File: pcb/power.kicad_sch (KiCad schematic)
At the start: 12 parts, among them P1 USB_C_Plug_USB2.0, U4 AZ1117IH-3.3TRG1

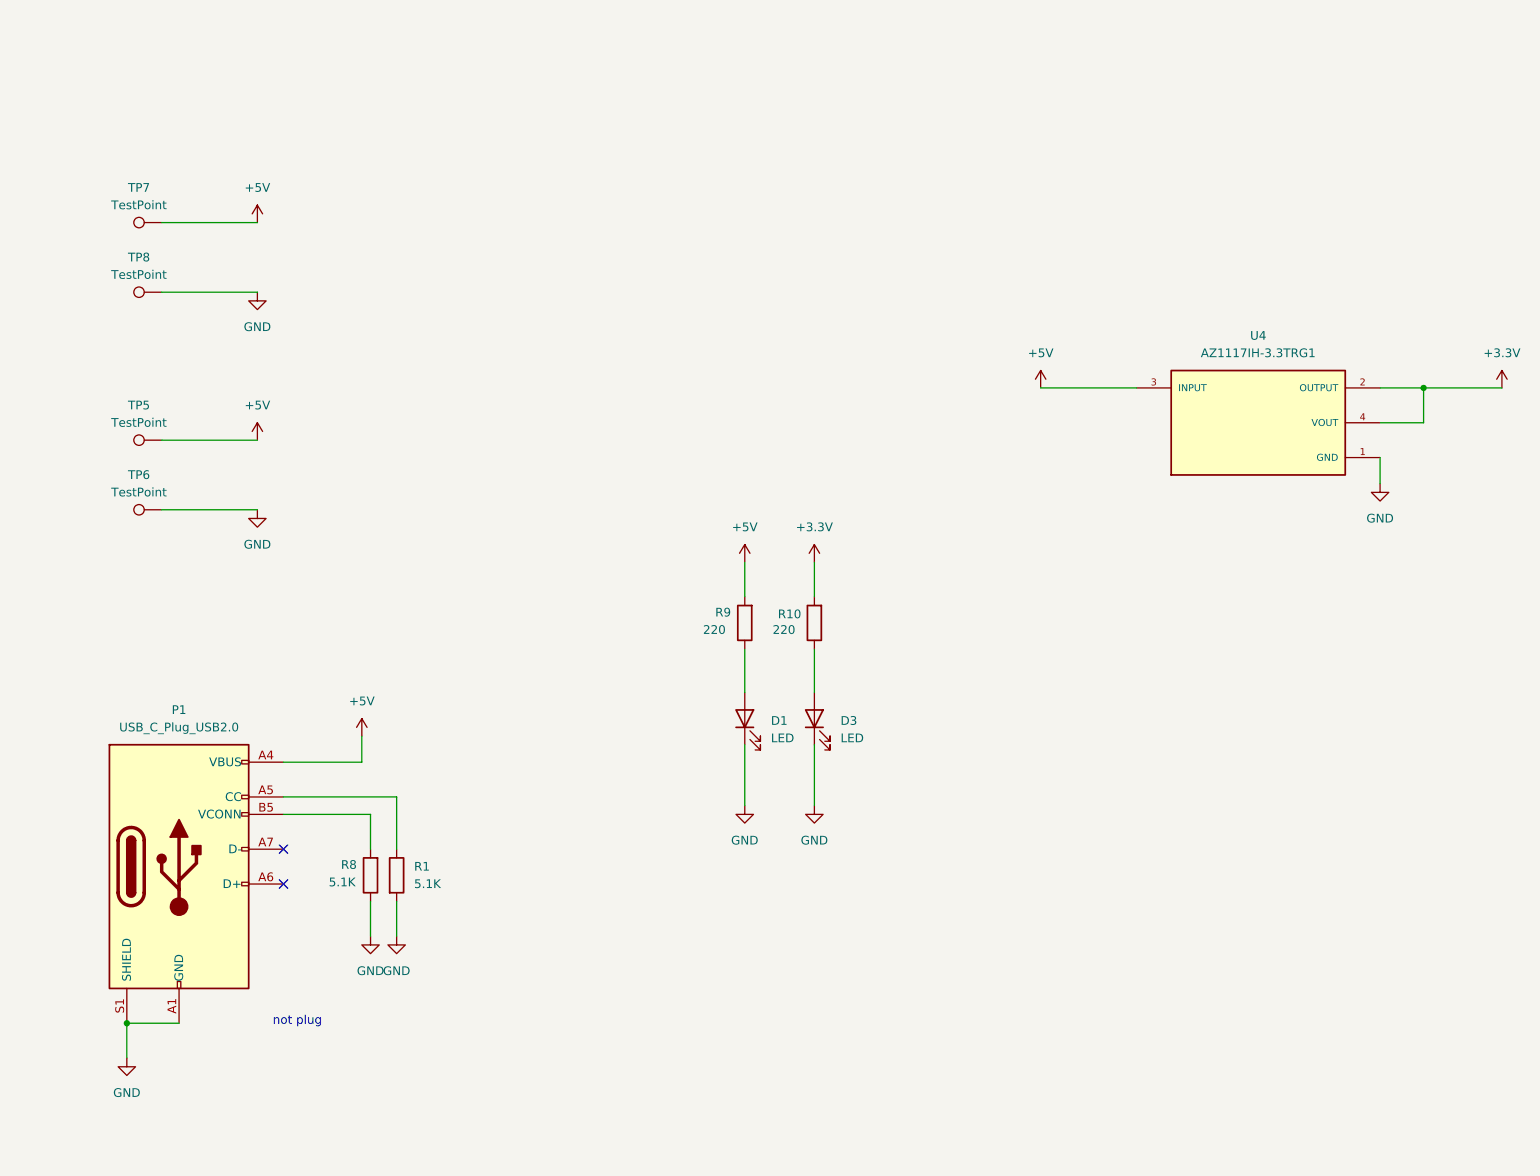
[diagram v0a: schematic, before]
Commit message: stuff
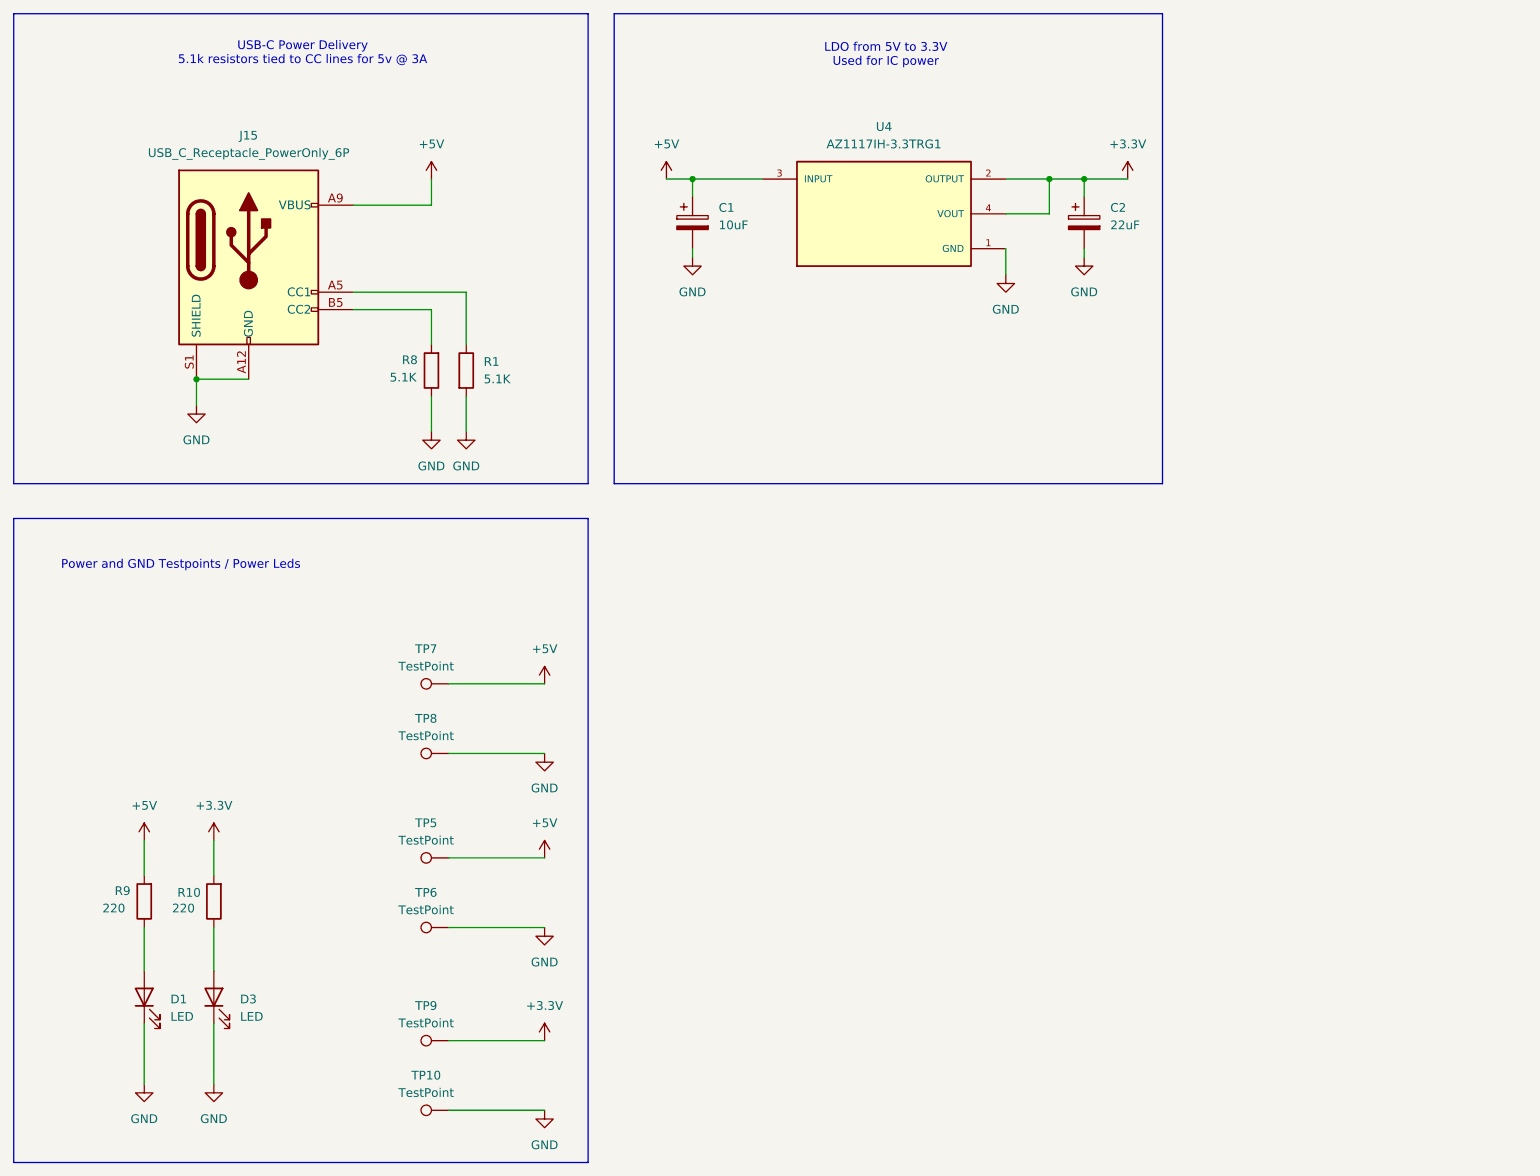
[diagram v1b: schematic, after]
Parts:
- removed P1: USB_C_Plug_USB2.0, symbol Connector:USB_C_Plug_USB2.0
- added C1: 10uF, Capacitor_SMD:C_0603_1608Metric, symbol Device:C_Polarized
- added C2: 22uF, Capacitor_SMD:C_0603_1608Metric, symbol Device:C_Polarized
- added J15: USB_C_Receptacle_PowerOnly_6P, Connector_USB:USB_C_Receptacle_GCT_USB4125-xx-x-0190_6P_TopMnt_Horizontal, symbol Connector:USB_C_Receptacle_PowerOnly_6P
- added TP10, TP9: TestPoint, TestPoint:TestPoint_Pad_3.0x3.0mm, symbol Connector:TestPoint
- D1, D3: footprint (none) -> LED_SMD:LED_0603_1608Metric
- R1, R10, R8, R9: footprint (none) -> Resistor_SMD:R_0603_1608Metric
- TP5, TP6, TP7, TP8: footprint (none) -> TestPoint:TestPoint_Pad_3.0x3.0mm
- U4: footprint AZ1117IH-3.3TRG1:SOT230P700X185-4N -> ldo:SOT230P700X185-4N
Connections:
- net +3.3V: now also C2.1, TP9.1
- net +5V: now also C1.1, J15.A9 (VBUS), J15.B9 (VBUS)
- net GND: now also C1.2, C2.2, J15.A12 (GND), J15.B12 (GND), J15.S1 (SHIELD), TP10.1
- net at R1.1: now also J15.A5 (CC1)
- net at R8.2: now also J15.B5 (CC2)
- no-connect marks 2 -> 0
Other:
- note added: "LDO from 5V to 3.3V Used for IC power"
- note added: "Power and GND Testpoints / Power Leds"
- note added: "USB-C Power Delivery 5.1k resistors tied to CC lines for 5v @ 3A"
- note removed: "not plug"
- moved on the sheet: D1, D3, R1, R10, R8, R9, TP5, TP6, TP7, TP8, U4
